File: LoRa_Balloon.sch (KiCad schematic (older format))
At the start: 13 parts, among them U2 SX1272IMLTRICT-ND_CID104

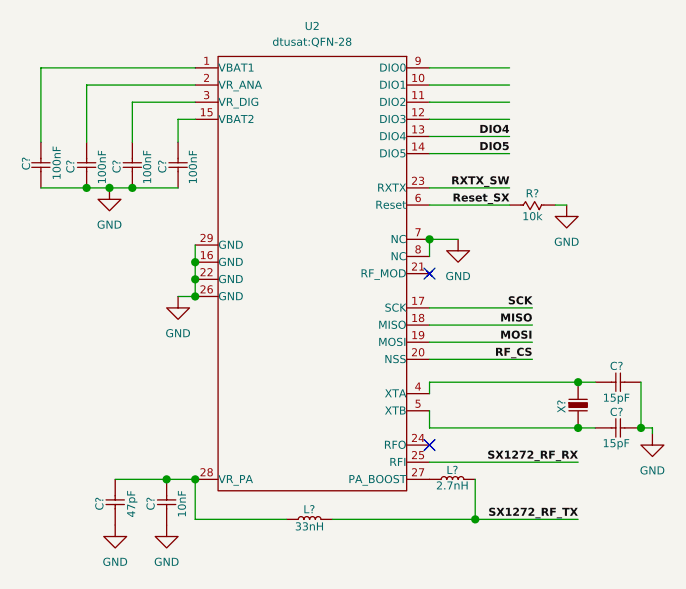
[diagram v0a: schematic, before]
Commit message: Add files via upload
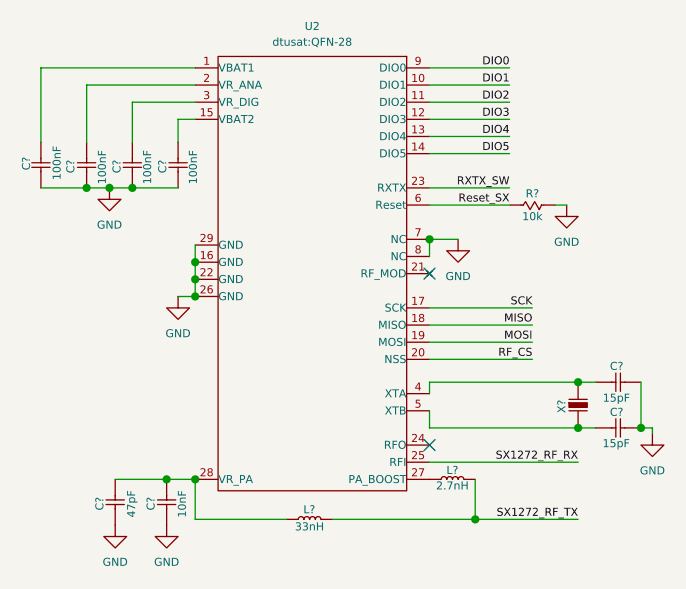
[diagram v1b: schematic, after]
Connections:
- net labels added: DIO0, DIO1, DIO2, DIO3
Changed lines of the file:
@@
 EESchema Schematic File Version 4
+LIBS:LoRa_Balloon-cache
 EELAYER 30 0
 EELAYER END
@@
 	1575 3250 1975 3250
 Connection ~ 1575 3075
-Text Label 3250 3000 2    35   ~ 7
+Text Label 3250 3000 2    35   ~ 0
 SX1272_RF_RX
 Wire Wire Line
@@
 Wire Wire Line
 	2800 3250 3250 3250
-Text Label 3250 3250 2    35   ~ 7
+Text Label 3250 3250 2    35   ~ 0
 SX1272_RF_TX
 Wire Wire Line
@@
 Wire Wire Line
 	2600 2325 3050 2325
-Text Label 3050 2550 2    35   ~ 7
+Text Label 3050 2550 2    35   ~ 0
 RF_CS
-Text Label 3050 2475 2    35   ~ 7
+Text Label 3050 2475 2    35   ~ 0
 MOSI
-Text Label 3050 2400 2    35   ~ 7
+Text Label 3050 2400 2    35   ~ 0
 MISO
-Text Label 3050 2325 2    35   ~ 7
+Text Label 3050 2325 2    35   ~ 0
 SCK
 $Comp
@@
 	2600 2100 2600 2025
 Connection ~ 2600 2025
-Text Label 2950 1800 2    35   ~ 7
+Text Label 2950 1800 2    35   ~ 0
 RXTX_SW
 $Comp
@@
 	0    1    1    0
 $EndComp
-Text Label 2950 1875 2    35   ~ 7
+Text Label 2950 1875 2    35   ~ 0
 Reset_SX
 Wire Wire Line
@@
 Wire Wire Line
 	2600 1275 2950 1275
-Text Label 2950 1650 2    35   ~ 7
+Text Label 2950 1650 2    35   ~ 0
 DIO5
-Text Label 2950 1575 2    35   ~ 7
+Text Label 2950 1575 2    35   ~ 0
 DIO4
+Text Label 2950 1500 2    35   ~ 0
+DIO3
+Text Label 2950 1425 2    35   ~ 0
+DIO2
+Text Label 2950 1350 2    35   ~ 0
+DIO1
+Text Label 2950 1275 2    35   ~ 0
+DIO0
 $EndSCHEMATC
